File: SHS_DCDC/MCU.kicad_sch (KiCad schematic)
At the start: 27 parts, among them J3 Conn_ARM_JTAG_SWD_10, J4 0022232041, J5 640456-2, SW1 TACT_SW, SW2 TACT_SW, SW3 TACT_SW, SW4 TACT_SW, SW5 TACT_SW, U8 MIC5501-3.0YM5, Y1 2-SMD no lead

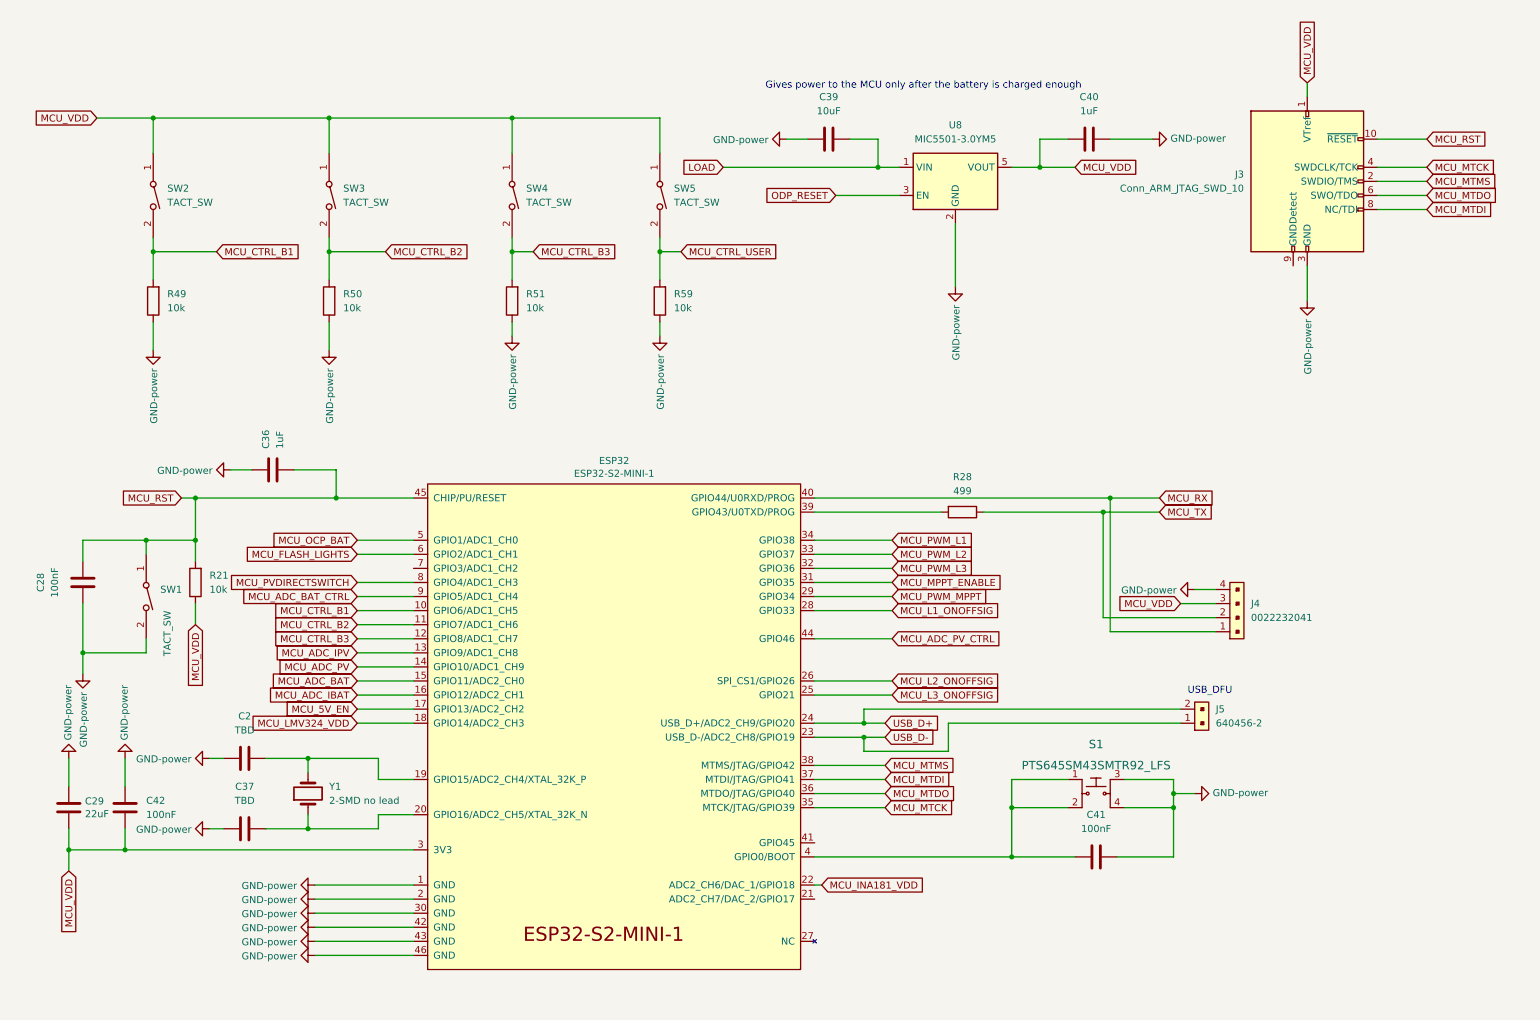
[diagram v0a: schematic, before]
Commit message: LED
Placement of the 2nd dual LED
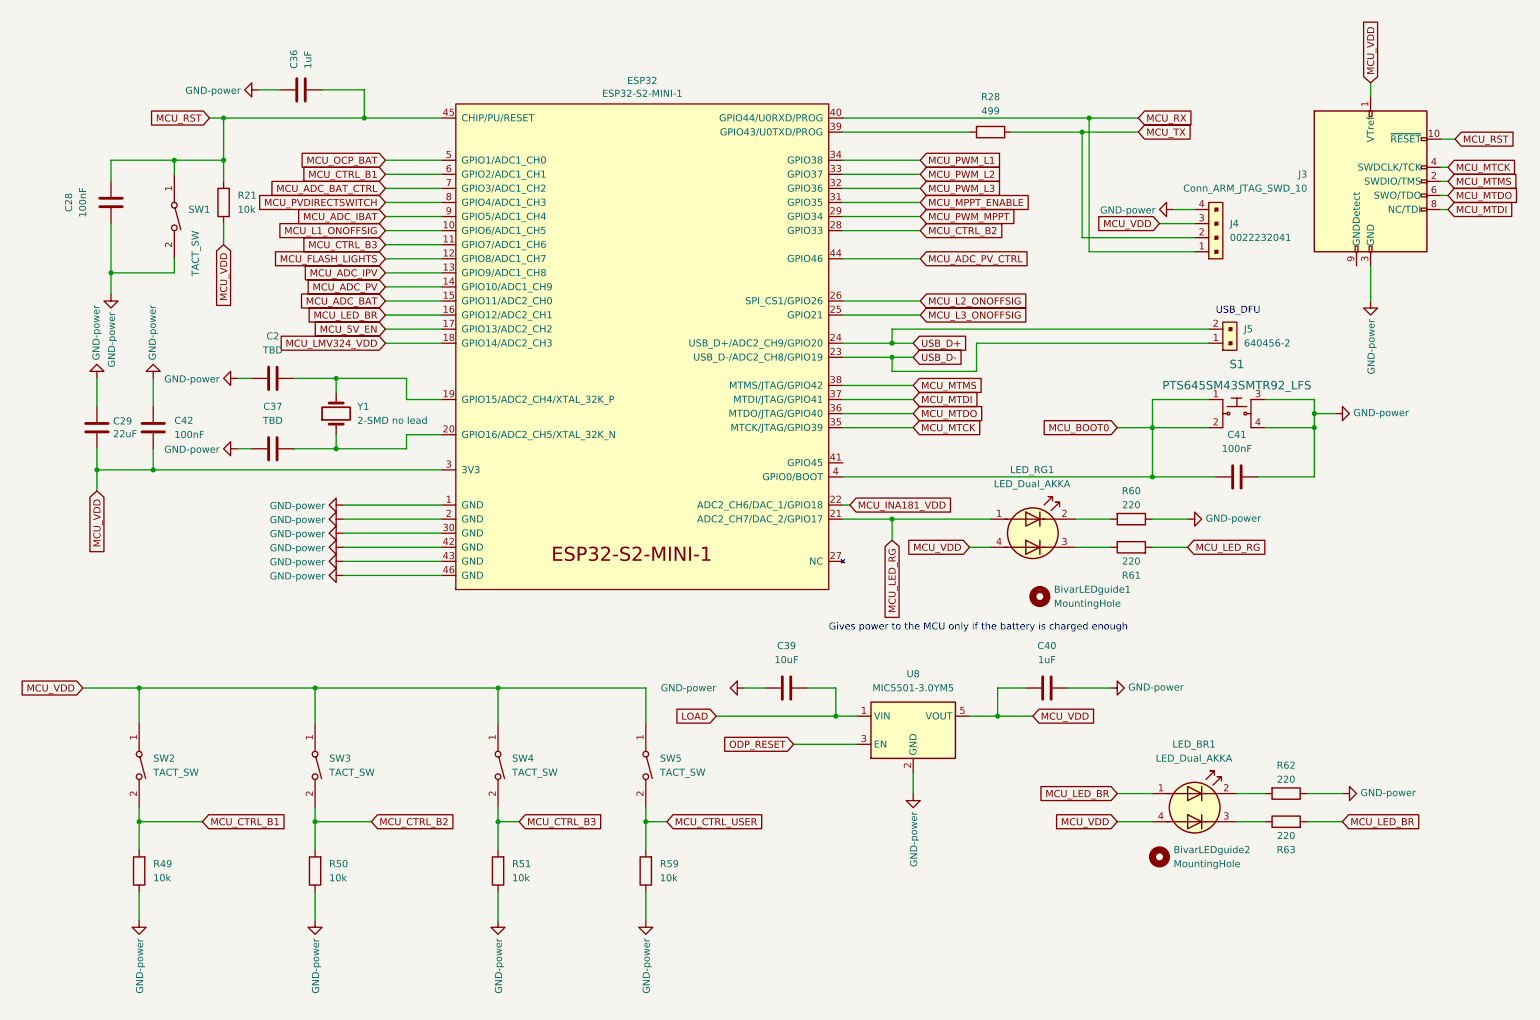
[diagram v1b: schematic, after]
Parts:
- added BivarLEDguide1, BivarLEDguide2: MountingHole, SHS_DCDC:BIVAR VLP-XXX-F, symbol Mechanical:MountingHole
- added LED_BR1, LED_RG1: LED_Dual_AKKA, LED_SMD:LED_Kingbright_APHBM2012_2x1.25mm, symbol Device:LED_Dual_AKKA
- added R60, R61, R62, R63: 220, Resistor_SMD:R_0402_1005Metric, symbol Device:R
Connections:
- net GND: now also R60.1, R62.1
- net MCU_ADC_BAT_CTRL: now also ESP32.7 (GPIO3/ADC1_CH2); no longer ESP32.9 (GPIO5/ADC1_CH4)
- net MCU_ADC_IBAT: now also ESP32.9 (GPIO5/ADC1_CH4); no longer ESP32.16 (GPIO12/ADC2_CH1)
- net MCU_CTRL_B1: now also ESP32.6 (GPIO2/ADC1_CH1); no longer ESP32.10 (GPIO6/ADC1_CH5)
- net MCU_CTRL_B2: now also ESP32.28 (GPIO33); no longer ESP32.11 (GPIO7/ADC1_CH6)
- net MCU_CTRL_B3: now also ESP32.11 (GPIO7/ADC1_CH6); no longer ESP32.12 (GPIO8/ADC1_CH7)
- net MCU_FLASH_LIGHTS: now also ESP32.12 (GPIO8/ADC1_CH7); no longer ESP32.6 (GPIO2/ADC1_CH1)
- net MCU_L1_ONOFFSIG: now also ESP32.10 (GPIO6/ADC1_CH5); no longer ESP32.28 (GPIO33)
- net MCU_VDD: now also LED_BR1.4 (A2), LED_RG1.4 (A2)
- net MCU_LED_RG: now reaches ESP32.21 (ADC2_CH7/DAC_2/GPIO17)
- net MCU_LED_RG: now also LED_RG1.1 (A1), R61.2
- net MCU_BOOT0: now reaches C41.2, ESP32.4 (GPIO0/BOOT), S1.1, S1.2
- new net: LED_BR1.3 (K2), R63.1
- new net: LED_RG1.2 (K1), R60.2
- new net: LED_BR1.2 (K1), R62.2
- new net: LED_RG1.3 (K2), R61.1
- new net MCU_LED_BR: ESP32.16 (GPIO12/ADC2_CH1), LED_BR1.1 (A1), R63.2
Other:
- note added: "Gives power to the MCU only if the battery is charged enough"
- note removed: "Gives power to the MCU only after the battery is charged enough"
- moved on the sheet: C2, C28, C29, C36, C37, C39, C40, C41, C42, ESP32, J3, J4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

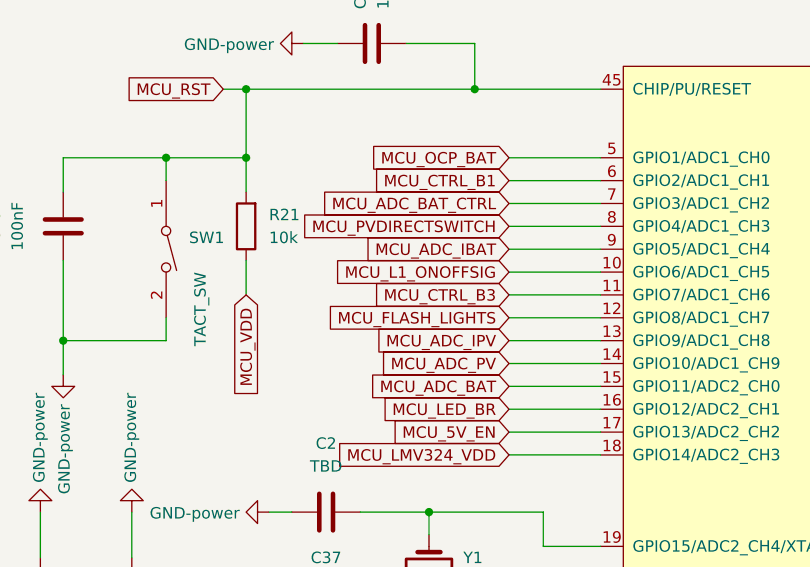
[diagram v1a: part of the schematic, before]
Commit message: Final_check stage
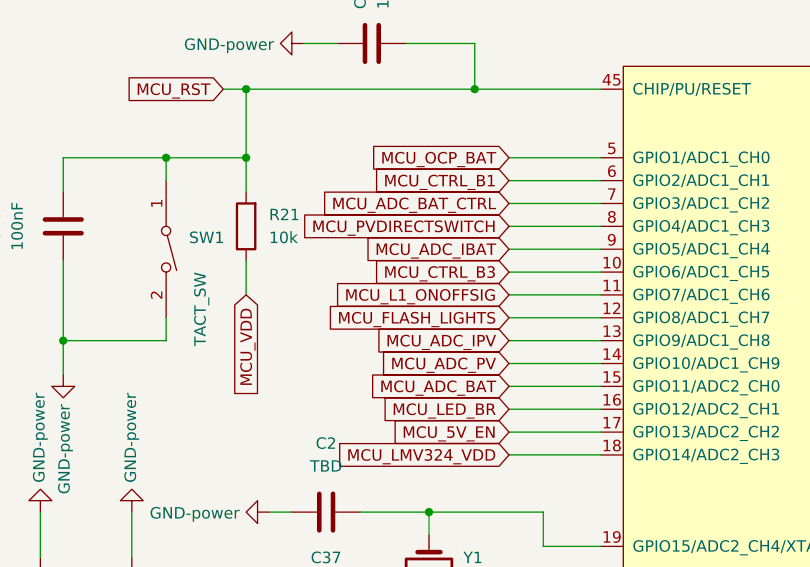
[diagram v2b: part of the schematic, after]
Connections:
- net MCU_CTRL_B3: now also ESP32.10 (GPIO6/ADC1_CH5); no longer ESP32.11 (GPIO7/ADC1_CH6)
- net MCU_L1_ONOFFSIG: now also ESP32.11 (GPIO7/ADC1_CH6); no longer ESP32.10 (GPIO6/ADC1_CH5)
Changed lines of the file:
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@@
     )
   )
-  (global_label "MCU_L1_ONOFFSIG" (shape input) (at 80.01 49.53 180) (fields_autoplaced)
+  (global_label "MCU_CTRL_B3" (shape input) (at 80.01 49.53 180) (fields_autoplaced)
     (effects (font (size 1.27 1.27)) (justify right))
-    (property "Intersheet References" "${INTERSHEET_REFS}" (id 0) (at 60.2082 49.6094 0)
+    (property "Intersheet References" "${INTERSHEET_REFS}" (id 0) (at 64.6834 49.4506 0)
       (effects (font (size 1.27 1.27)) (justify right) hide)
     )
@@
     )
   )
-  (global_label "MCU_CTRL_B3" (shape input) (at 80.01 52.07 180) (fields_autoplaced)
+  (global_label "MCU_L1_ONOFFSIG" (shape input) (at 80.01 52.07 180) (fields_autoplaced)
     (effects (font (size 1.27 1.27)) (justify right))
-    (property "Intersheet References" "${INTERSHEET_REFS}" (id 0) (at 64.6834 51.9906 0)
+    (property "Intersheet References" "${INTERSHEET_REFS}" (id 0) (at 60.2082 51.9906 0)
       (effects (font (size 1.27 1.27)) (justify right) hide)
     )
